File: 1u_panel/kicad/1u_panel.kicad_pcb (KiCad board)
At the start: 2 copper layers, 83 x 100 mm, 112 parts, among them J1 SAMTEC-MMS-104-02-X-SHJ, J2 ORESAT-DEBUG-CONNECTOR-ALL, Q1 MOSFET-PCH-SOT23-6, Q2 MOSFET-PCH-SOT23-6, U1 TCAN330, U10 TPS63060, U11 TMP101NA/3KSLOTTED, U12 LTC4412, U2 TMP101NA/3KSLOTTED, U3 LT1618EMSTRPBF, U4 INA226AIDGSR, U7 STM32F091C, X1 16MHZ-2.5x2mm

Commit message: Cleaned up schematic; added correct values and part numbers, added datasheet links to important components, imported sch to brd, LOTS of errors to clean up there but it's at synced now.
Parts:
- CELL1, CELL2: value XTE-SF 27.7cm2 -> SPECTROLAB-XTE-SF
- CF1: value HARWIN M55-6021242R -> M55-6021242R
- D5: value MBR0520L -> NRVB130TGSOD123
- J1: value SAMTEC-MMS-104-02-X-SHJ -> MMS-104-01-[F/L]-SH
- J2: value ORESAT-DEBUG-CONNECTOR-ALL -> 2-1734592-0
- L1: value 1 uH -> 1u
- Q1: value MOSFET-PCH-SOT23-6 -> DMP3050LVT-7
- Q2: value MOSFET-PCH-SOT23-6 -> DMP2240UDM-7
- U1: value TCAN330 -> TCAN330GDCNT
- U10: value TPS63060 -> TPS63060DSCR
- U7: value STM32F091C -> STM32F091CCT7
- X1: value 16MHZ-2.5x2mm -> ECS-160-10-36Q-ES-TR
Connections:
- net 4412-CTL renamed Net-(U12-CTL)
- net 4412-GATE renamed Net-(Q2A-G)
- net AUX renamed Net-(CF1-AUX-Pad7)
- net BOOT0 renamed /Microcontroller/BOOT0
- net CAN_RX renamed /Microcontroller/CAN_RX
- net CAN_SHDN renamed /Microcontroller/CAN_SHDN
- net CAN_SILENT renamed /Microcontroller/CAN_SILENT
- net CAN_TX renamed /Microcontroller/CAN_TX
- net DEBU-1/SOLAR3V renamed Net-(J2-DEBUG-1)
- net DEBUG-0 renamed Net-(J2-DEBUG-0)
- net DEBUG-2 renamed Net-(J2-DEBUG-2)
- net DEBUG-3 renamed Net-(J2-DEBUG-3)
- net INTERCELL renamed Net-(CELL1-A1)
- net LT1618-FB renamed Net-(U3-FB)
- net LT1618-ISN renamed Net-(L2-1)
- net LT1618-SW renamed Net-(D5-ANODE)
- net LT1618-VC renamed Net-(U3-VC)
- net NRESET renamed /Microcontroller/NRESET
- net PA0 renamed /Microcontroller/PA0
- net PA2/USART2_TX renamed /Microcontroller/PA2/USART2_TX
- net PA3/USART2_RX renamed /Microcontroller/PA3/USART2_RX
- net PA5 renamed Net-(U7-PA5)
- net PA6 renamed Net-(U7-PA6)
- net SMSN0 renamed /Microcontroller/SMSN0
- net SMSN1 renamed /Microcontroller/SMSN1
- net SMSN2 renamed /Microcontroller/SMSN2
- net SMSN3 renamed /Microcontroller/SMSN3
- net SWCLK renamed /Microcontroller/SWCLK
- net SWDIO renamed /Microcontroller/SWDIO
- net SWO renamed Net-(J2-SWO)
- net TPS-EN renamed Net-(U10-PS/SYNC)
- net TPS-FB renamed Net-(U10-FB)
- net TPS-L1 renamed Net-(U10-L1)
- net TPS-L2 renamed Net-(U10-L2)
- net TPS-PG renamed Net-(U10-PG)
- net TPS-VAUX renamed Net-(U10-VAUX)
- net TPS-VIN renamed Net-(U10-VIN)
- net TPS-VOUT-3.3V renamed /MPPT / PWR/TPS-VOUT-3.3V
- net VMPPT renamed /MPPT / PWR/VMPPT
- net XTAL1-IN renamed Net-(U7-PF0-OSC_IN)
- net XTAL1-OUT renamed Net-(U7-PF1-OSC_OUT)
- net ~{SHDN-3.3V} renamed /MPPT / PWR/~{SHDN-3.3V}
- net ~{SHDN-OUPUT} renamed /MPPT / PWR/~{SHDN-OUPUT}
- net ~{SHUTDOWN} renamed /MPPT / PWR/~{SHUTDOWN}
- J2 pad 4: (no net) -> unconnected-(J2-DEVICE-D+-Pad4)
- J2 pad 5: (no net) -> unconnected-(J2-DEVICE-D--Pad5)
- J2 pad 7: (no net) -> unconnected-(J2-HOST-D+-Pad7)
- J2 pad 8: (no net) -> unconnected-(J2-HOST-D--Pad8)
- U7 pad 17: (no net) -> unconnected-(U7-PA7-Pad17)
- U7 pad 18: (no net) -> unconnected-(U7-PB0-Pad18)
- U7 pad 19: (no net) -> unconnected-(U7-PB1-Pad19)
- U7 pad 2: (no net) -> unconnected-(U7-PC13-Pad2)
- U7 pad 20: (no net) -> unconnected-(U7-PB2-Pad20)
- U7 pad 29: (no net) -> unconnected-(U7-PA8-Pad29)
- U7 pad 3: (no net) -> unconnected-(U7-PC14-OSC32_IN-Pad3)
- U7 pad 38: (no net) -> unconnected-(U7-PA15-Pad38)
- U7 pad 39: (no net) -> unconnected-(U7-PB3-Pad39)
- U7 pad 4: (no net) -> unconnected-(U7-PC15-OSC32_OUT-Pad4)
- U7 pad 40: (no net) -> unconnected-(U7-PB4-Pad40)
- U7 pad 41: (no net) -> unconnected-(U7-PB5-Pad41)
- U7 pad 42: (no net) -> unconnected-(U7-PB6-Pad42)
- U7 pad 43: (no net) -> unconnected-(U7-PB7-Pad43)
- U7 pad 45: (no net) -> unconnected-(U7-PB8-Pad45)
- U7 pad 46: (no net) -> unconnected-(U7-PB9-Pad46)

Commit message: Switch to PSAS naming convention!
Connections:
- net /MPPT / PWR/TPS-VOUT-3.3V renamed /1u_panel-power/TPS-VOUT-3.3V
- net /MPPT / PWR/VMPPT renamed /1u_panel-power/VMPPT
- net /MPPT / PWR/~{SHDN-3.3V} renamed /1u_panel-power/~{SHDN-3.3V}
- net /MPPT / PWR/~{SHDN-OUPUT} renamed /1u_panel-power/~{SHDN-OUPUT}
- net /MPPT / PWR/~{SHUTDOWN} renamed /1u_panel-power/~{SHUTDOWN}
- net /Microcontroller/BOOT0 renamed /1u_panel-microcontroller/BOOT0
- net /Microcontroller/CAN_RX renamed /1u_panel-microcontroller/CAN_RX
- net /Microcontroller/CAN_SHDN renamed /1u_panel-microcontroller/CAN_SHDN
- net /Microcontroller/CAN_SILENT renamed /1u_panel-microcontroller/CAN_SILENT
- net /Microcontroller/CAN_TX renamed /1u_panel-microcontroller/CAN_TX
- net /Microcontroller/NRESET renamed /1u_panel-microcontroller/NRESET
- net /Microcontroller/PA0 renamed /1u_panel-microcontroller/PA0
- net /Microcontroller/PA2/USART2_TX renamed /1u_panel-microcontroller/PA2/USART2_TX
- net /Microcontroller/PA3/USART2_RX renamed /1u_panel-microcontroller/PA3/USART2_RX
- net /Microcontroller/SMSN0 renamed /1u_panel-microcontroller/SMSN0
- net /Microcontroller/SMSN1 renamed /1u_panel-microcontroller/SMSN1
- net /Microcontroller/SMSN2 renamed /1u_panel-microcontroller/SMSN2
- net /Microcontroller/SMSN3 renamed /1u_panel-microcontroller/SMSN3
- net /Microcontroller/SWCLK renamed /1u_panel-microcontroller/SWCLK
- net /Microcontroller/SWDIO renamed /1u_panel-microcontroller/SWDIO

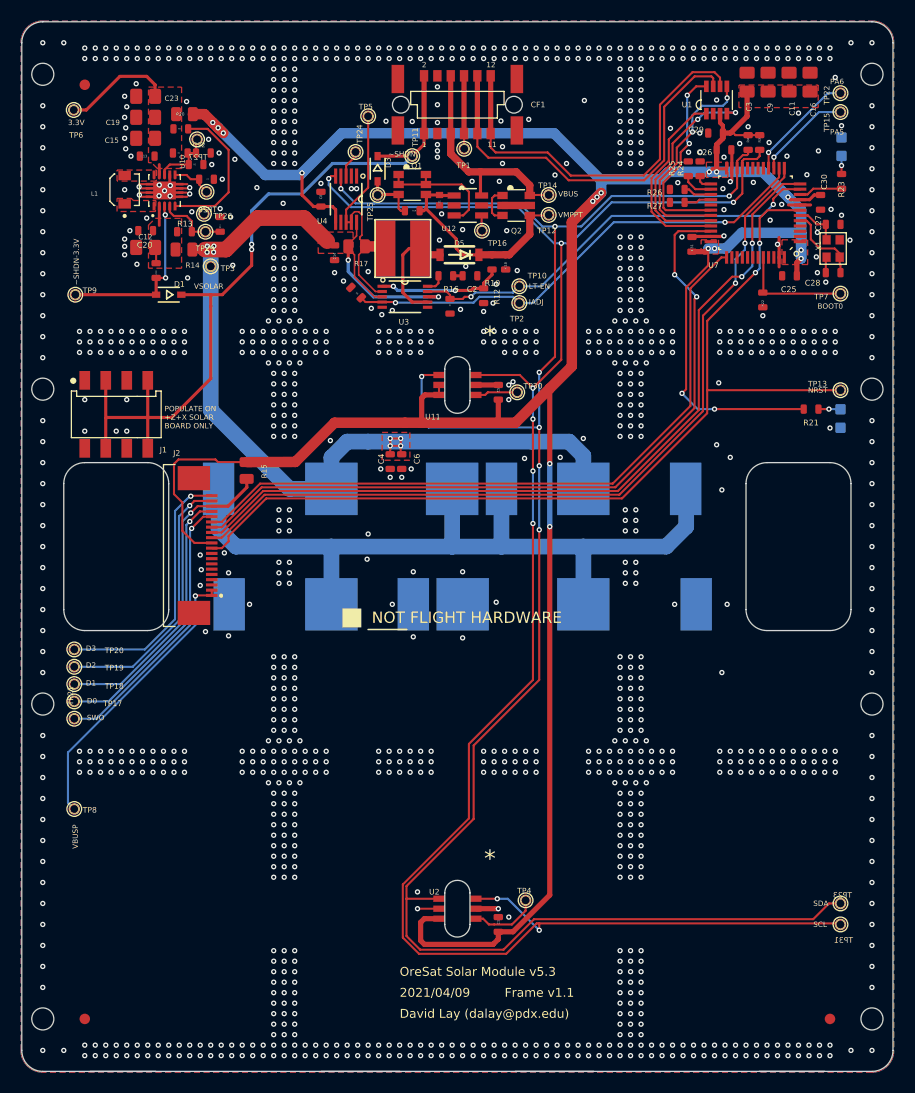
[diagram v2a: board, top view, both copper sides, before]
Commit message: Beginning of the v6.0 solar boards. Lots of ways to go.
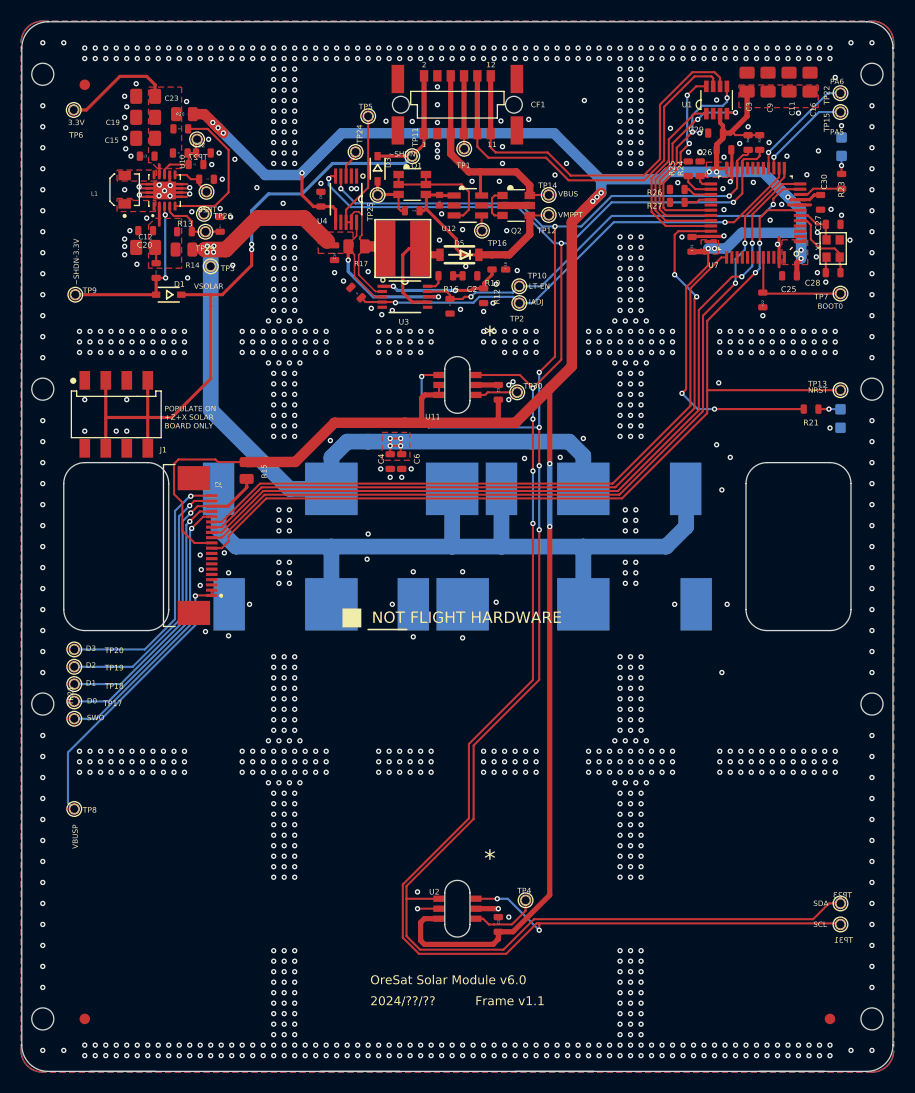
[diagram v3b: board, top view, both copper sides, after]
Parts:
- J2: footprint 1u_panel:TE_2-1734592-0 -> oresat-connectors:J-TE-2-1734592-0
- R12: value 14.2k -> 14.7k
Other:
- outline, holes or cut-outs redrawn
- board text added: "2024/??/??"
- board text added: "Frame v2.0"
- board text added: "OreSat Solar Module v6.0"
- board text removed: "2021/04/09"
- board text removed: "David Lay (dalay@pdx.edu)"
- board text removed: "OreSat Solar Module v5.3"
